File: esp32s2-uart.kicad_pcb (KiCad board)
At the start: 2 copper layers, 44.2 x 14.7 mm, 38 parts, among them J1 USB_C_Receptacle_USB2.0, J2 Conn_01x06, J3 Conn_02x04_Odd_Even, U1 AMS1117-3.3, U2 ESP32-S2FH4, Y1 Crystal_GND24_Small

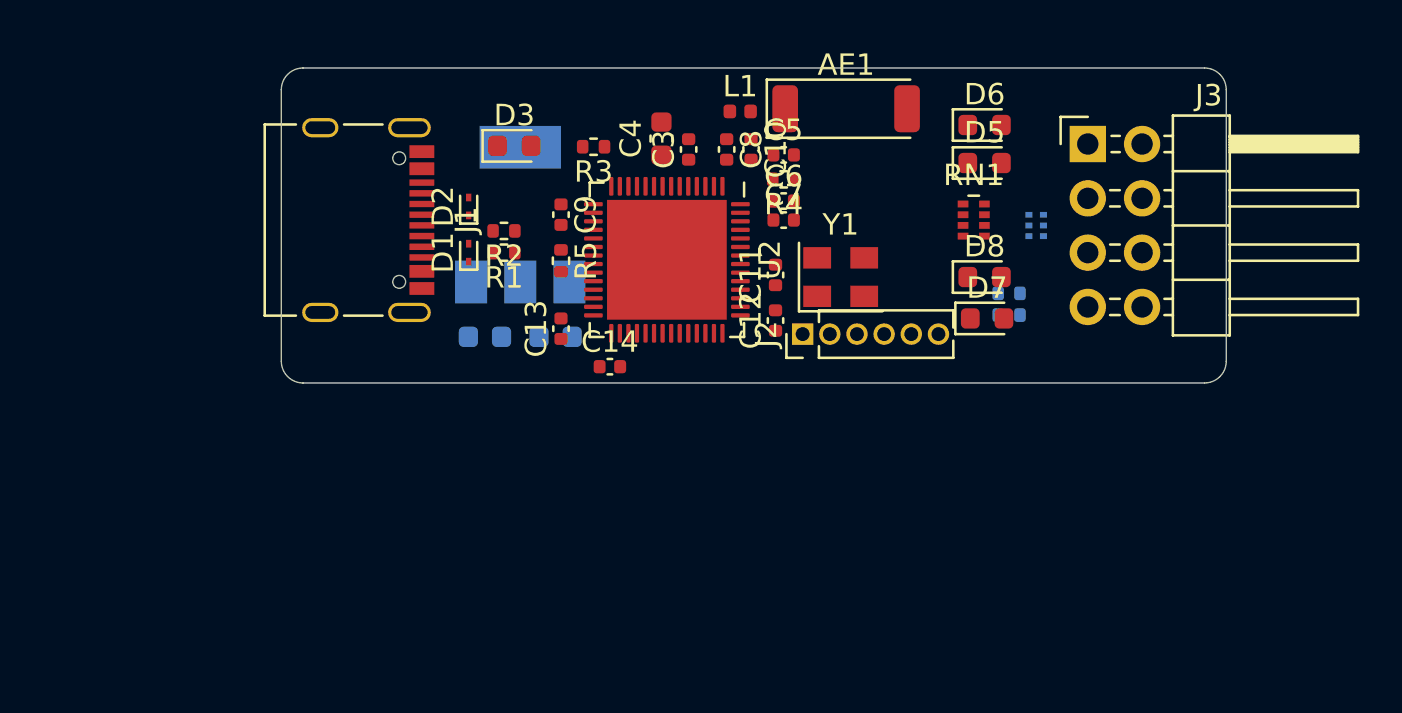
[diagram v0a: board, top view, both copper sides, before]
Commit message: update
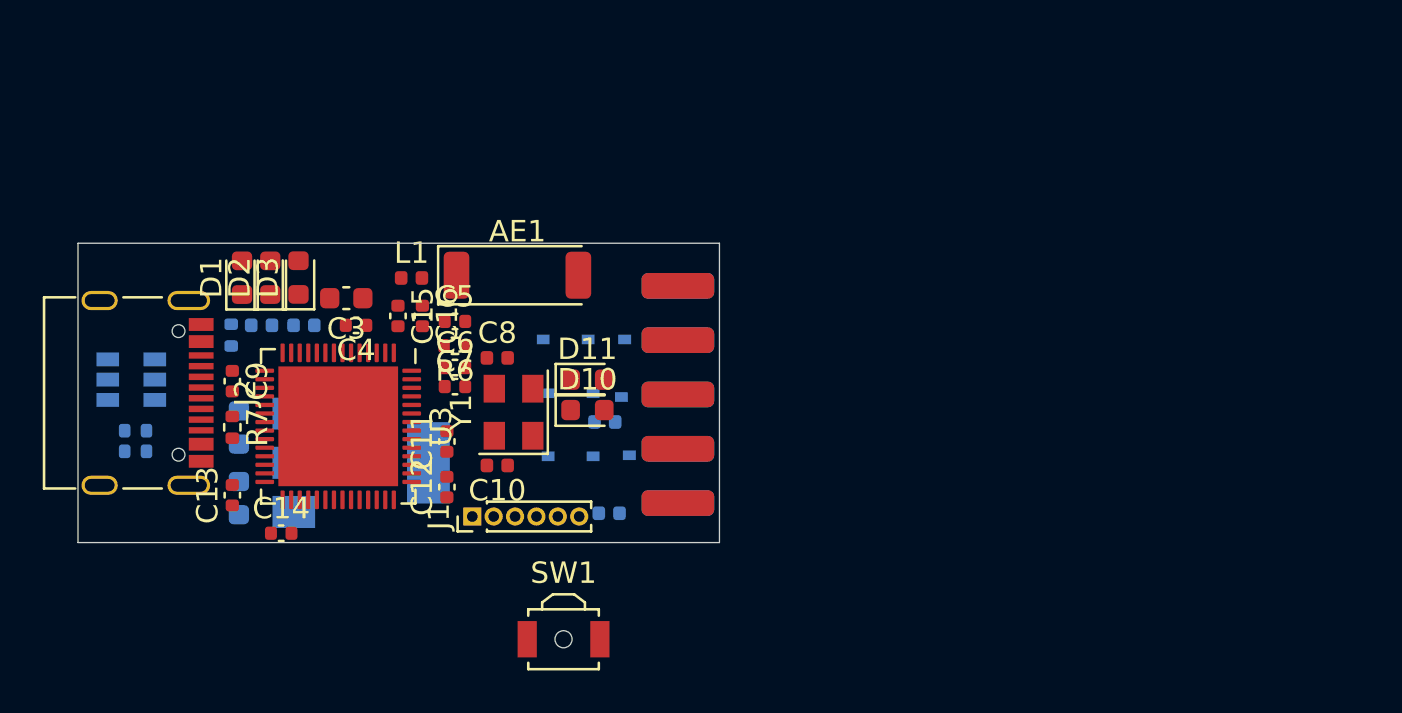
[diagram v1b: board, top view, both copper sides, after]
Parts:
- removed the J1 at (131.6, 89.9)
- removed the R5 at (140.6, 91.8)
- removed RN1: 2.2k, Resistor_SMD:R_Array_Concave_4x0402
- added C15: TBD, Capacitor_SMD:C_0402_1005Metric, F.Cu at (133.0, 94.4)
- added C16: TBD, Capacitor_SMD:C_0402_1005Metric, F.Cu at (134.1, 94.4)
- added D1: RED, LED_SMD:LED_0603_1608Metric, F.Cu at (125.7, 92.6)
- added D8: PESD5V0S1BA, Diode_SMD:D_SOD-323, B.Cu at (144.8, 100.9)
- added D9: PESD5V0S1BA, Diode_SMD:D_SOD-323, B.Cu at (144.6, 95.5)
- added J2: USB_C_Receptacle_USB2.0, Connector_USB:USB_C_Receptacle_Palconn_UTC16-G, F.Cu at (121.3, 98.0)
- added R3: 1k, Resistor_SMD:R_0402_1005Metric, B.Cu at (128.6, 94.8)
- added R8: 1k, Resistor_SMD:R_0402_1005Metric, B.Cu at (142.8, 103.6)
- added R9: 1k, Resistor_SMD:R_0402_1005Metric, B.Cu at (142.6, 99.4)
- added SW1: SW_Push, Button_Switch_SMD:SW_SPST_B3U-3000P-B, F.Cu at (140.7, 109.5)
- added U3: ESP32-S2FH4, Package_DFN_QFN:QFN-56-1EP_7x7mm_P0.4mm_EP5.6x5.6mm, F.Cu at (130.2, 99.6)
- C10, C8: value TBD -> 10pf
- C2: value 4.7uf -> 10uf
- C3: value 0.1uf -> 10uf; footprint Capacitor_SMD:C_0402_1005Metric -> Capacitor_SMD:C_0603_1608Metric
- C4: value 10uf -> 0.1uf; footprint Capacitor_SMD:C_0603_1608Metric -> Capacitor_SMD:C_0402_1005Metric
- D2: value ESD9B3.3ST5G -> GREEN; footprint Diode_SMD:D_SOD-923 -> LED_SMD:LED_0603_1608Metric
- D3: value LED -> BLUE
- D4: value PESD3V3L4UF -> PESD5V0S1BA; footprint Package_TO_SOT_SMD:SOT-886 -> Diode_SMD:D_SOD-323
- D5, D6: value LED -> PESD5V0S1BA; footprint LED_SMD:LED_0603_1608Metric -> Diode_SMD:D_SOD-323; moved to B.Cu
- D7: renamed from D1; value ESD9B3.3ST5G -> PESD5V0S1BA; footprint Diode_SMD:D_SOD-923 -> Diode_SMD:D_SOD-323; moved to B.Cu
- J1: renamed from J2; footprint Connector_PinHeader_1.27mm:PinHeader_1x06_P1.27mm_Vertical -> Connector_PinHeader_1.00mm:PinHeader_1x06_P1.00mm_Vertical
- J3: value Conn_02x04_Odd_Even -> Conn_02x05_Counter_Clockwise; footprint Connector_PinHeader_2.54mm:PinHeader_2x04_P2.54mm_Horizontal -> my_footprint:Header_2x5_pin
- R1, R2: moved to B.Cu
- R4: value 10k -> 1k; moved to B.Cu
- R5: renamed from R3; moved to B.Cu
- R6: value 0 -> 10k; moved to F.Cu
- R7: value NC -> 10k; moved to F.Cu
- U2: value ESP32-S2FH4 -> USBLC6-2SC6; footprint Package_DFN_QFN:QFN-56-1EP_7x7mm_P0.4mm_EP5.6x5.6mm -> Package_TO_SOT_SMD:SOT-23-6; moved to B.Cu
- moved R7 36.9 mm to (125.2, 99.6), turned to 270 degrees
- moved R6 26.0 mm to (135.6, 95.8), turned to 180 degrees
- moved U2 25.7 mm to (120.5, 97.4), turned to 180 degrees
- moved R4 25.4 mm to (126.6, 94.8)
- moved D4 24.3 mm to (141.0, 101.0)
- moved D6 23.1 mm to (141.0, 98.0)
- moved J3 20.3 mm to (146.1, 93.0)
- moved R2 20.1 mm to (120.7, 100.7)
- moved D5 19.3 mm to (144.5, 98.2)
- moved D11 19.2 mm to (141.8, 97.4)
- moved D10 19.2 mm to (141.8, 98.8)
- moved R1 19.1 mm to (120.7, 99.8)
- moved R5 19.1 mm to (125.2, 95.3), turned to 90 degrees
- moved C10 19.0 mm to (137.6, 101.4), turned to 180 degrees
- moved J1 17.7 mm to (136.4, 103.8)
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- renumbered D7 to D10, D8 to D11
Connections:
- C10 pad 1: Net-(AE1-Pad1) -> Net-(C10-Pad1)
- C8 pad 1: /LNA_IN -> Net-(C8-Pad1)
- D10 pad 2: /VOUT -> +5V
- D11 pad 2: /VOUT -> +5V
- D2 pad 1: Net-(D2-Pad1) -> GND
- D2 pad 2: GND -> Net-(D2-Pad2)
- D4 pad 1: /UART_RX -> /IO0_TMS
- D5 pad 1: Net-(D5-Pad1) -> /CTS_TDI
- D5 pad 2: /VOUT -> GND
- D6 pad 1: Net-(D6-Pad1) -> /RTS_TDO
- D6 pad 2: /VOUT -> GND
- D7 pad 2: Net-(D1-Pad2) -> /UART_TX
- J3 pad 1: /IO0 -> /IO0_TMS
- J3 pad 2: /UART_TX -> /CTS_TDI
- J3 pad 3: /EN -> /RTS_TDO
- J3 pad 4: /UART_RX -> +3V3
- J3 pad 5: /RTS -> +5V
- J3 pad 6: /CTS -> GND
- J3 pad 7: /VOUT -> GND
- J3 pad 8: GND -> /EN_TCK
- R1 pad 2: Net-(D1-Pad2) -> Net-(R1-Pad2)
- R2 pad 2: Net-(D2-Pad1) -> Net-(R2-Pad2)
- R4 pad 1: +3V3 -> Net-(R4-Pad1)
- R4 pad 2: /DBG_EN -> Net-(D2-Pad2)
- R5 pad 1: Net-(R3-Pad1) -> Net-(R5-Pad1)
- R6 pad 2: /VOUT -> /DBG_EN
- R7 pad 1: +5V -> +3V3
- R7 pad 2: /VOUT -> Net-(R7-Pad2)
- U2 pad 1: +3V3 -> Net-(J2-PadA7)
- U2 pad 2: /LNA_IN -> GND
- U2 pad 3: +3V3 -> Net-(J2-PadA6)
- U2 pad 4: +3V3 -> Net-(R2-Pad2)
- U2 pad 5: /DBG_IO0 -> +5V
- U2 pad 6: Net-(U2-Pad6) -> Net-(R1-Pad2)
- Y1 pad 1: Net-(U2-Pad52) -> Net-(C10-Pad1)
- Y1 pad 3: Net-(U2-Pad53) -> Net-(C8-Pad1)
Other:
- board size 44.2 x 14.7 mm -> 30 x 14 mm
